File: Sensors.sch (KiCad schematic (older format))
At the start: 18 parts, among them P10 CONN_01X03, P11 CONN_01X03, P12 CONN_01X03, P13 CONN_01X03, Q9 FDN340P, U5 MCP9700

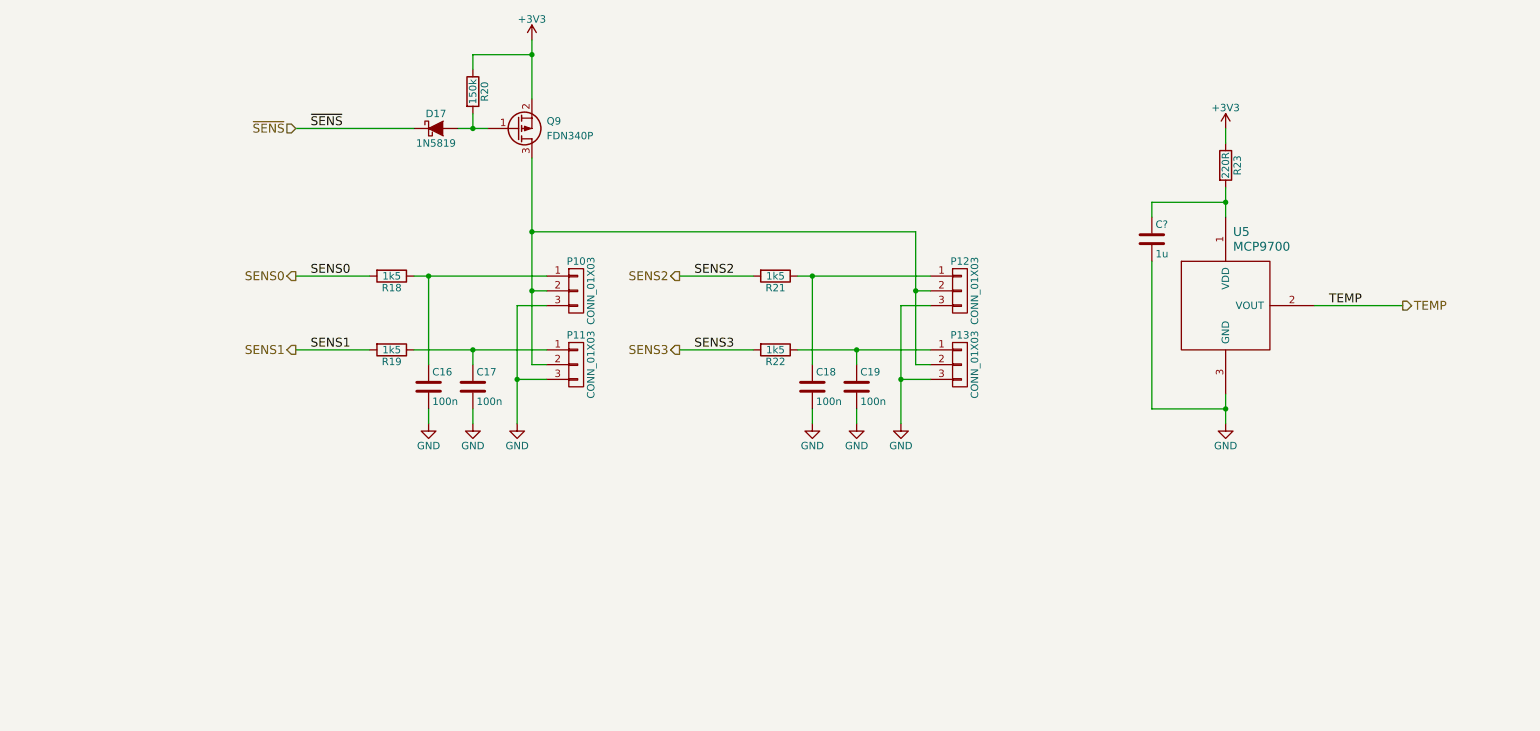
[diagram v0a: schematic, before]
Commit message: Finished schematics
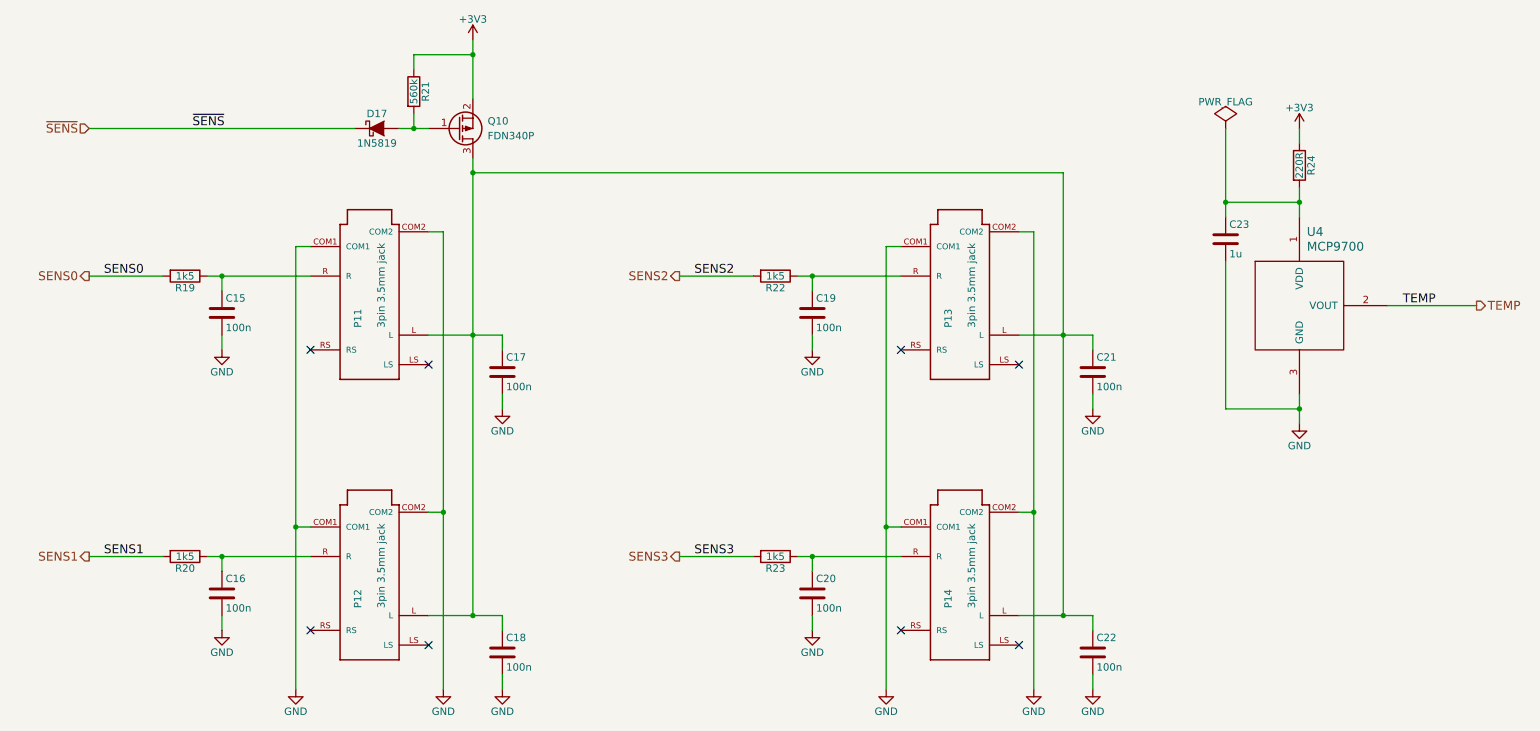
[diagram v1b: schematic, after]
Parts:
- removed P10, P11, P12, P13: CONN_01X03, symbol CONN_01X03
- removed R20: 150k, symbol R
- added C17, C20, C21, C22: 100n, Capacitors_SMD:C_0603, symbol C
- added P11, P12, P13, P14: 3pin 3.5mm jack, jakub:SUNTECH_ST-PJ-312, symbol ST-PJ-312
- added R23: 1k5, Resistors_SMD:R_0603, symbol R
- C15: renamed from C16; footprint (none) -> Capacitors_SMD:C_0603
- C16: renamed from C17; footprint (none) -> Capacitors_SMD:C_0603
- C18, C19: footprint (none) -> Capacitors_SMD:C_0603
- C23: renamed from C?; footprint (none) -> Capacitors_SMD:C_0603
- D17: footprint (none) -> Diodes_SMD:SMA_Standard
- Q10: renamed from Q9; footprint (none) -> TO_SOT_Packages_SMD:SOT-23
- R19: renamed from R18; footprint (none) -> Resistors_SMD:R_0603
- R20: renamed from R19; footprint (none) -> Resistors_SMD:R_0603
- R21: value 1k5 -> 560k; footprint (none) -> Resistors_SMD:R_0603; Alt. Order Code 301010114 -> 301010230; Note 1.5kΩ/1% 0603 resistor -> 560kΩ/5% 0603 resistor; Order Code 9233407 -> 9233717; Part Number RC0603JR-071K5L -> RC0603JR-07560KL
- R22: footprint (none) -> Resistors_SMD:R_0603
- R24: renamed from R23; footprint (none) -> Resistors_SMD:R_0603
- U4: renamed from U5; footprint (none) -> TO_SOT_Packages_SMD:SOT-23
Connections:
- net +3V3: now also R21.1
- net GND: now also C17.2, C20.2, C21.2, C22.2, P11.COM1, P11.COM2, P12.COM1, P12.COM2, P13.COM1, P13.COM2, P14.COM1, P14.COM2
- net SENS2: now also R22.2; no longer R21.2
- net SENS3: now also R23.2; no longer R22.2
- net at C15.1, R19.1: now also P11.R
- net at Q10.3 (D): now also C18.1, C17.1, C21.1, C22.1, P11.L, P12.L, P13.L, P14.L
- net at C16.1, R20.1: now also P12.R
- net at C19.1, R22.1: now also P13.R
- net at D17.2 (A), Q10.1 (G): now also R21.2
- new net: C20.1, P14.R, R23.1
- no-connect marks 0 -> 8
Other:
- moved on the sheet: C15, C16, C23, D17, Q10, R19, R20, R24, U4
